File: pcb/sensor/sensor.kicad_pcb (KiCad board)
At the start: 2 copper layers, 45 x 40 mm, 10 parts, among them J1 Conn_01x02, U1 MOUDLE-SEEEDUINO-XIAO-ESP32C3, U4 DHT11

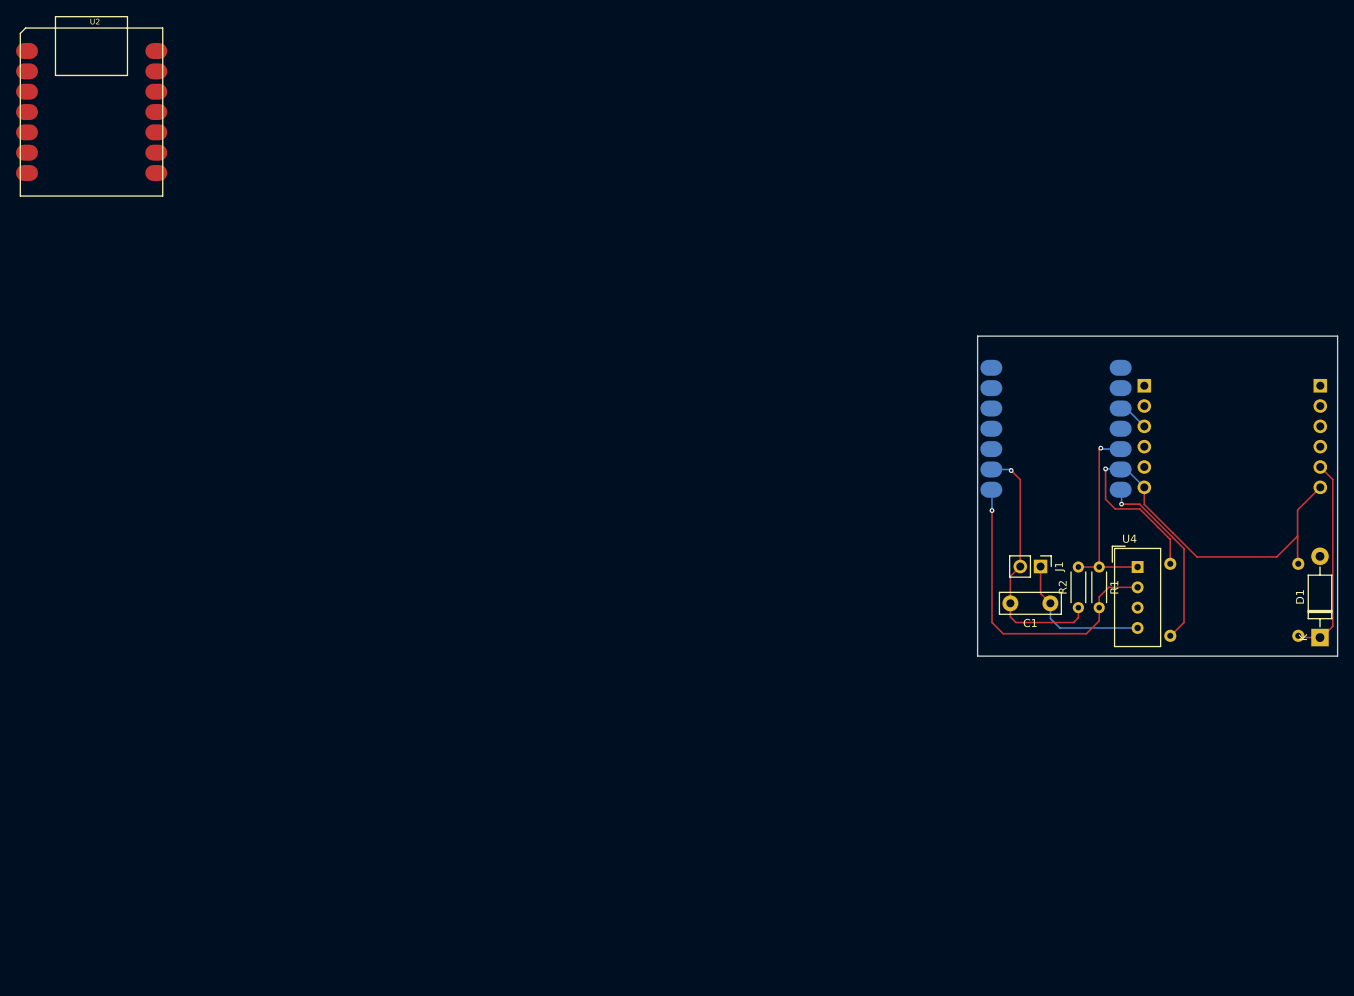
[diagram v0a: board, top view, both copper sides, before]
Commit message: PCB ready
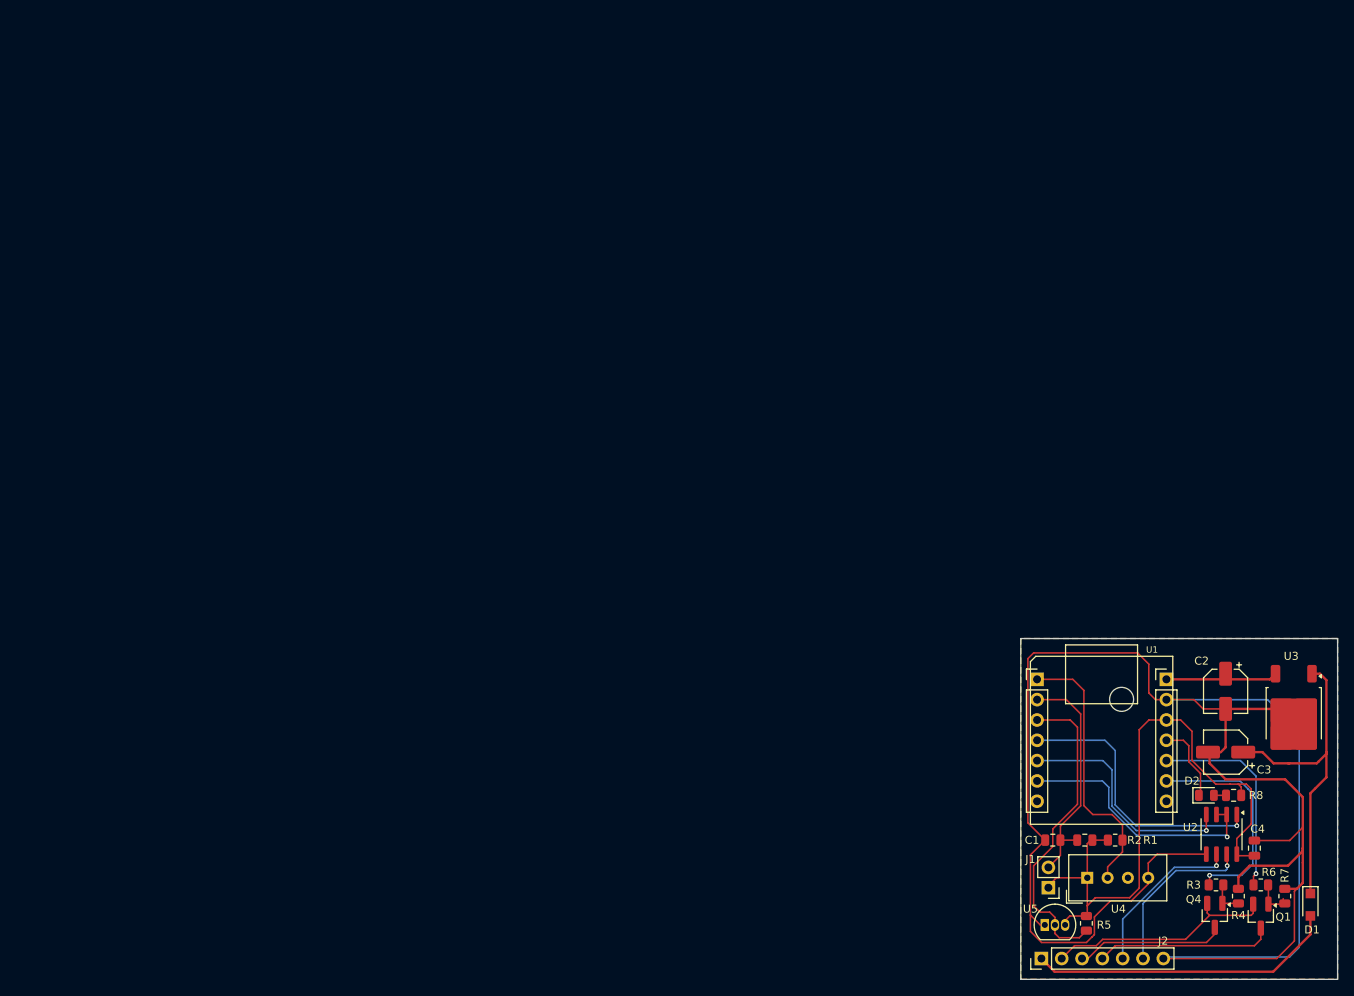
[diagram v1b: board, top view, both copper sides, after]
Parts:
- added C2: 100u, Capacitor_SMD:CP_Elec_5x5.4, F.Cu at (151.2, 84.4)
- added C3: 100u, Capacitor_SMD:CP_Elec_5x5.4, F.Cu at (151.2, 92.0)
- added C4: 100n, Capacitor_SMD:C_0805_2012Metric, F.Cu at (154.8, 104.0)
- added D2: LED, LED_SMD:LED_0805_2012Metric, F.Cu at (148.8, 97.4)
- added J2: Conn_01x07, Connector_PinHeader_2.54mm:PinHeader_1x07_P2.54mm_Vertical, F.Cu at (128.2, 117.8)
- added Q1: Q_NMOS, Package_TO_SOT_SMD:SOT-23_Handsoldering, F.Cu at (155.6, 112.5)
- added Q4: Q_NMOS, Package_TO_SOT_SMD:SOT-23_Handsoldering, F.Cu at (149.8, 112.4)
- added R3: 1k, Resistor_SMD:R_0805_2012Metric, F.Cu at (150.0, 108.6)
- added R4: 33k, Resistor_SMD:R_0805_2012Metric, F.Cu at (152.8, 110.0)
- added R5: 4.7k, Resistor_SMD:R_0805_2012Metric, F.Cu at (133.8, 113.4)
- added R6: 1k, Resistor_SMD:R_0805_2012Metric, F.Cu at (155.6, 108.6)
- added R7: 33k, Resistor_SMD:R_0805_2012Metric, F.Cu at (158.6, 110.0)
- added R8: 470, Capacitor_SMD:C_0805_2012Metric, F.Cu at (152.2, 97.4)
- added REF**: MountingHole_3mm, MountingHole:MountingHole_3mm, F.Cu at (138.2, 85.4)
- C1: footprint Capacitor_THT:C_Disc_D7.5mm_W2.5mm_P5.00mm -> Capacitor_SMD:C_0805_2012Metric
- D1: footprint Diode_THT:D_DO-41_SOD81_P10.16mm_Horizontal -> Diode_SMD:Nexperia_CFP3_SOD-123W
- R1: footprint Resistor_THT:R_Axial_DIN0204_L3.6mm_D1.6mm_P5.08mm_Horizontal -> Resistor_SMD:R_0805_2012Metric
- R2: footprint Resistor_THT:R_Axial_DIN0204_L3.6mm_D1.6mm_P5.08mm_Horizontal -> Capacitor_SMD:C_0805_2012Metric
- U1: moved to F.Cu
- U2: value ~ -> SP3485CN; footprint seedstudio:MOUDLE14P-SMD-2.54-21X17.8MM -> Package_SO:SOIC-8_3.9x4.9mm_P1.27mm
- U3: value ~ -> L7805; footprint seedstudio:Optoisolator_HW399 -> Package_TO_SOT_SMD:TO-252-2; moved to F.Cu
- U5: value ~ -> DS18B20; footprint seedstudio:DCDC_HW187 -> Package_TO_SOT_THT:TO-92_Inline; moved to F.Cu
- moved U2 170.0 mm to (150.7, 102.3), turned to -90 degrees
- moved U1 60.2 mm to (126.8, 101.0)
- moved U5 56.8 mm to (128.6, 113.6), turned to 0 degrees
- moved U3 43.1 mm to (159.7, 87.2), turned to -90 degrees
- moved J1 40.2 mm to (129.1, 108.9), turned to 180 degrees
- moved U4 39.4 mm to (133.9, 107.7), turned to 90 degrees
- moved R1 34.2 mm to (137.4, 103.0), turned to 0 degrees
- moved D1 33.4 mm to (161.8, 111.1), turned to -90 degrees
- moved C1 29.6 mm to (129.6, 103.0)
- moved R2 29.1 mm to (133.6, 103.0), turned to 180 degrees
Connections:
- C1 pad 1: /GND -> /ADC_In
- C1 pad 2: /ADC_In -> GND
- D1 pad 2: /24V_IN -> +24V
- J1 pad 1: /GND -> 3.3V
- R1 pad 1: /3.3V -> 3.3V
- R2 pad 1: /ADC_In -> 3.3V
- R2 pad 2: /3.3V -> /ADC_In
- U1 pad 10: Net-(U1-PA5_A9_D9_MISO) -> /LIGHT_TRIG
- U1 pad 11: unconnected-(U1-PA6_A10_D10_MOSI-Pad11) -> Net-(D2-K)
- U1 pad 12: /3.3V -> 3.3V
- U1 pad 13: /GND -> GND
- U1 pad 3: unconnected-(U1-PA10_A2_D2-Pad3) -> /TEMP_SENS_1_WIRE
- U1 pad 4: unconnected-(U1-PA11_A3_D3-Pad4) -> /RS_RX
- U1 pad 5: unconnected-(U1-PA8_A4_D4_SDA-Pad5) -> /RS_TX
- U1 pad 6: unconnected-(U1-PA9_A5_D5_SCL-Pad6) -> /RS_RE_DE
- U1 pad 9: unconnected-(U1-PA7_A8_D8_SCK-Pad9) -> /AUX_TRIG
- U2 pad 1: unconnected-(U2-D0-Pad1) -> /RS_RX
- U2 pad 2: unconnected-(U2-D1-Pad2) -> /RS_RE_DE
- U2 pad 3: unconnected-(U2-D2-Pad3) -> /RS_RE_DE
- U2 pad 4: unconnected-(U2-D3-Pad4) -> /RS_TX
- U2 pad 5: unconnected-(U2-D4-Pad5) -> GND
- U2 pad 6: unconnected-(U2-D5-Pad6) -> /RS_A
- U2 pad 7: /UART_Tx -> /RS_B
- U2 pad 8: /UART_Rx -> 3.3V
- U3 pad 1: unconnected-(U3-OUT1-Pad1) -> Net-(D1-K)
- U3 pad 2: unconnected-(U3-OUT2-Pad2) -> GND
- U3 pad 3: unconnected-(U3-OUT3-Pad3) -> /5V
- U4 pad 1: /3.3V -> 3.3V
- U4 pad 4: /GND -> GND
- U5 pad 1: /GND -> GND
- U5 pad 2: /5V -> /TEMP_SENS_1_WIRE
- U5 pad 3: Net-(D1-K) -> 3.3V
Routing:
- net GND: track 0.00 -> 245.1 mm
- net 3.3V: track 0.00 -> 82.4 mm
- net /GND: track 78.6 -> 0.00 mm, vias 1 -> 0
- net /TEMP_SENS_1_WIRE: track 0.00 -> 39.8 mm
- net +24V: track 0.00 -> 38.6 mm
- net /RS_RX: track 0.00 -> 34.8 mm, vias 0 -> 1
- net /RS_RE_DE: track 0.00 -> 32.2 mm, vias 0 -> 1
- net /RS_TX: track 0.00 -> 29.5 mm, vias 0 -> 1
- net PLC_COM: track 0.00 -> 29.0 mm
- net /AUX_TRIG: track 0.00 -> 27.5 mm, vias 0 -> 1
- net /LIGHT_TRIG: track 0.00 -> 25.7 mm, vias 0 -> 1
- net /3.3V: track 25.2 -> 0.00 mm, vias 1 -> 0
- net /LIGHT_OUT: track 0.00 -> 22.4 mm
- net /RS_B: track 0.00 -> 21.1 mm, vias 0 -> 1
- net /RS_A: track 0.00 -> 20.9 mm, vias 0 -> 1
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- added copper zone on B.Cu, net GND
- added copper zone on F.Cu, net GND
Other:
- board size 45 x 40 mm -> 39.6 x 42.6 mm
